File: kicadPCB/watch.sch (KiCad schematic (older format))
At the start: 62 parts, among them IC1 ISL1209, J1 USB_OTG, M1 BOS_LIBS_SWD_BREAKOUTS, T1 BC850, U2 MKL27Z256VLH4, Y1 Crystal

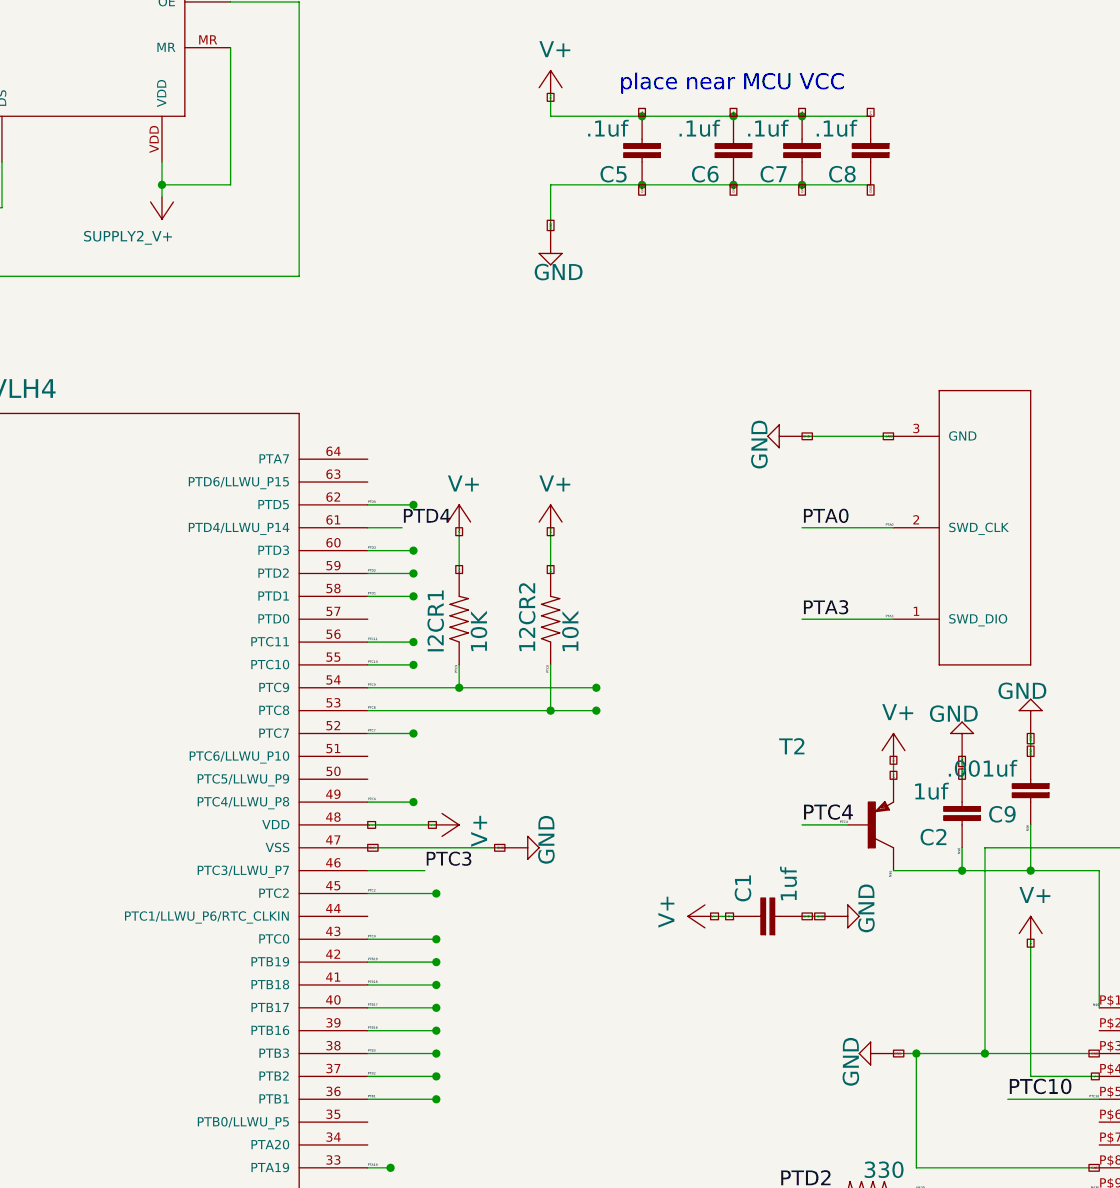
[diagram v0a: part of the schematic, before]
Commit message: fixed pnp
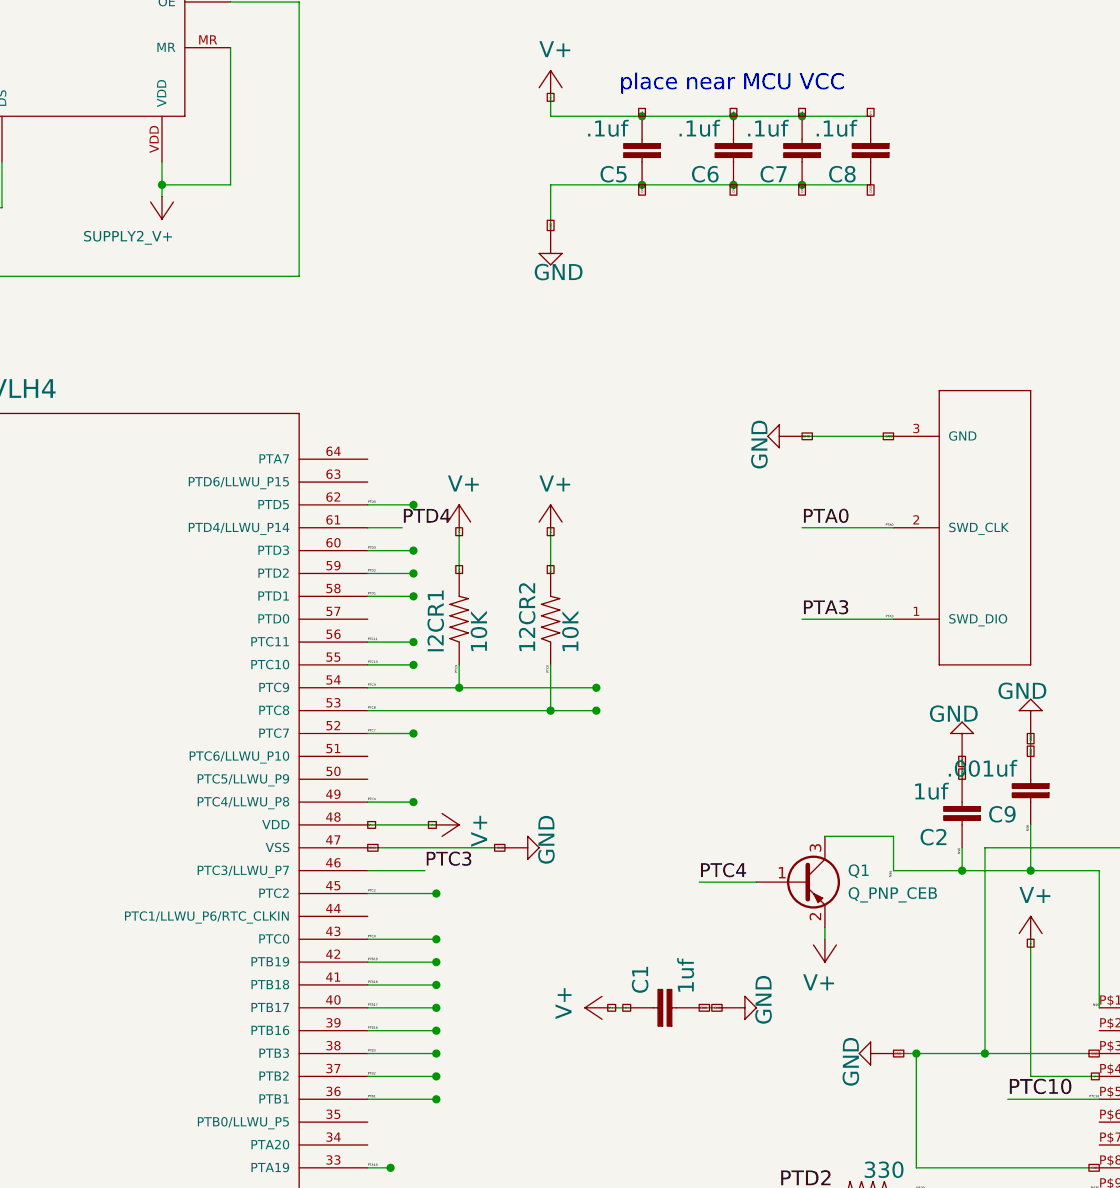
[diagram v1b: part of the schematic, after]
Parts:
- removed T2: ~, watch:TRANSISTOR_SOT23-EBC, symbol TRANSISTOR_-PNP-
- added Q1: Q_PNP_CEB, TO_SOT_Packages_SMD:SOT-23, symbol Q_PNP_BEC
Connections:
- net N$6: now also Q1.3 (C)
- net PTC4: now also Q1.1 (B)
- net V+: now also Q1.2 (E)
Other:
- moved on the sheet: C1
